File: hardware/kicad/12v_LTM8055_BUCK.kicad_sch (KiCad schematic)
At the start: 20 parts, among them U44 MCP4725A0T-E/CH, U47 LTM8055IY_PBF

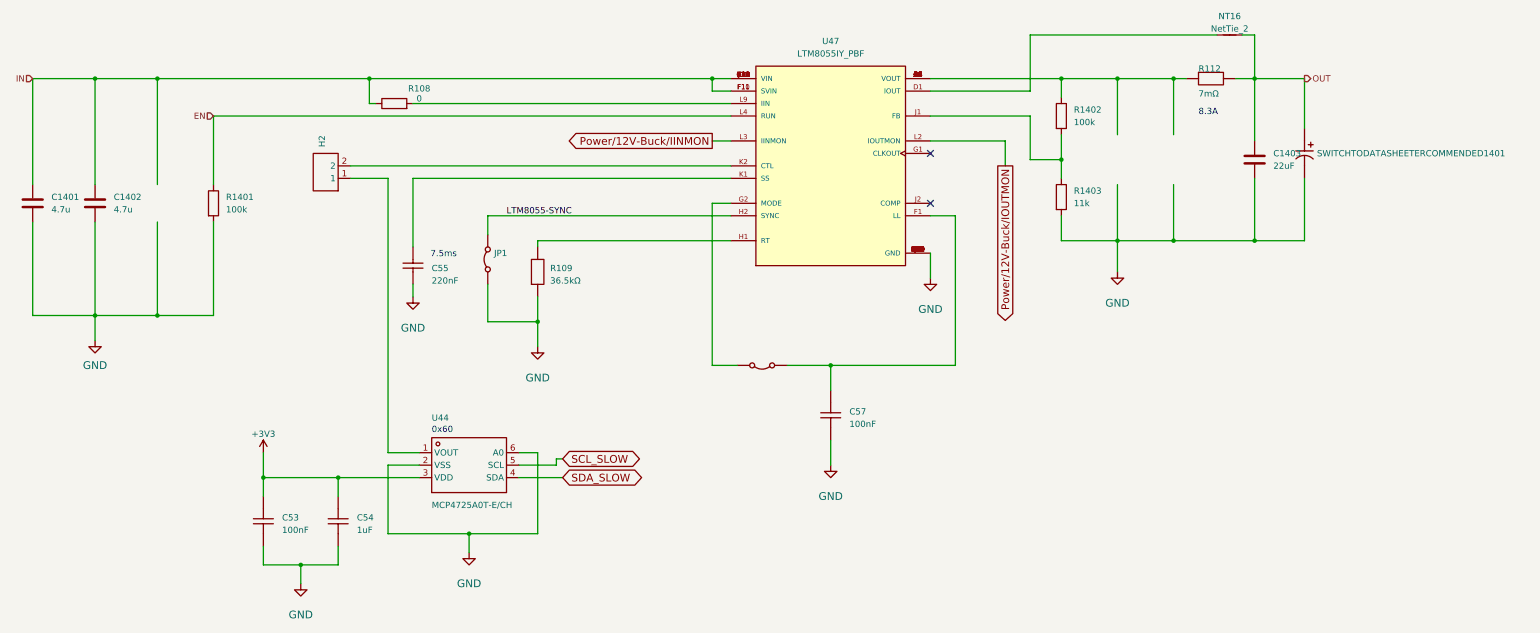
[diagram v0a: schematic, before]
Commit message: almost done 12v buck
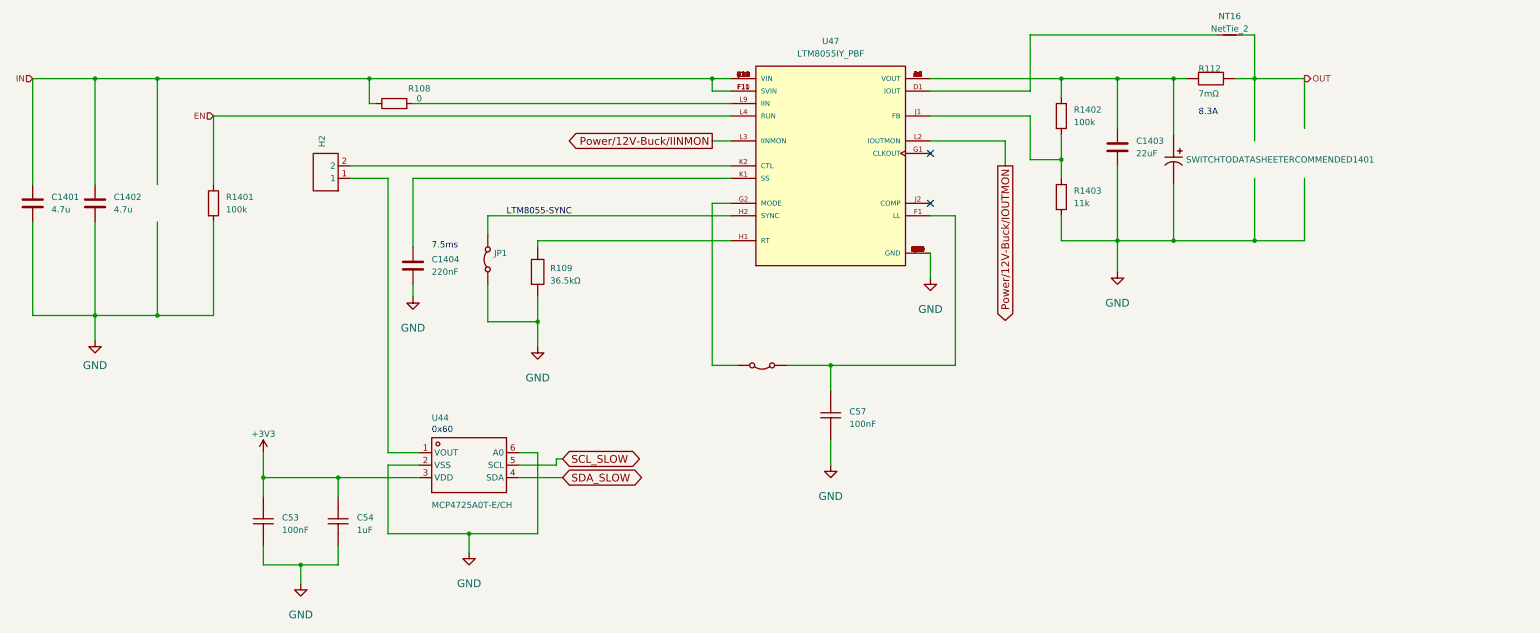
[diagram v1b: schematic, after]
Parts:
- removed C55: 220nF, 5v rail sm-easyedapro:C0603, symbol 5v rail sm-easyedapro:CL10B224KB8NNNC
- added C1404: 220nF, Capacitor_SMD:C_0402_1005Metric, symbol Device:C
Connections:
- net GND: now also C1404.2
- net OUT: no longer C1403.1, SWITCHTODATASHEETERCOMMENDED1401.1
- net at U47.K1 (SS): now also C1404.1
- net at R112.1, R1402.1, U47.A1 (VOUT)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: now also C1403.1, SWITCHTODATASHEETERCOMMENDED1401.1
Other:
- moved on the sheet: C1403, SWITCHTODATASHEETERCOMMENDED1401
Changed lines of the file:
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@@
 	(text "7.5ms"
 		(exclude_from_sim no)
-		(at 98.806 102.616 0)
+		(at 99.06 100.838 0)
 		(effects
 			(font
@@
 	(wire
 		(pts
-			(xy 238.76 87.63) (xy 238.76 99.06)
+			(xy 238.76 83.82) (xy 238.76 99.06)
 		)
 		(stroke
@@
 	(wire
 		(pts
-			(xy 238.76 66.04) (xy 238.76 77.47)
+			(xy 238.76 66.04) (xy 238.76 76.2)
 		)
 		(stroke
@@
 	)
 	(symbol
-		(lib_id "5v rail sm-easyedapro:CL10B224KB8NNNC")
-		(at 95.25 104.14 90)
-		(unit 1)
-		(exclude_from_sim no)
-		(in_bom yes)
-		(on_board yes)
-		(dnp no)
-		(property "Reference" "C55"
-			(at 99.06 105.41 90)
-			(effects
-				(font
-					(size 1.27 1.27)
-				)
-				(justify right top)
-			)
-		)
-		(property "Value" "220nF"
-			(at 99.06 107.95 90)
-			(effects
-				(font
-					(size 1.27 1.27)
-				)
-				(justify right top)
-			)
-		)
-		(property "Footprint" "5v rail sm-easyedapro:C0603"
-			(at 95.25 104.14 0)
-			(effects
-				(font
-					(size 1.27 1.27)
-				)
-				(hide yes)
-			)
-		)
-		(property "Datasheet" "https://item.szlcsc.com/datasheet/CL10B224KB8NNNC/65773.html"
-			(at 95.25 104.14 0)
-			(effects
-				(font
-					(size 1.27 1.27)
-				)
-				(hide yes)
-			)
-		)
-		(property "Description" "Capacitance:220nF Tolerance:±10% Tolerance:±10% Voltage Rating:50V Temperature Coefficient:X7R"
-			(at 95.25 104.14 0)
-			(effects
-				(font
-					(size 1.27 1.27)
-				)
-				(hide yes)
-			)
-		)
-		(property "Manufacturer Part" "CL10B224KB8NNNC"
-			(at 95.25 104.14 0)
-			(effects
-				(font
-					(size 1.27 1.27)
-				)
-				(hide yes)
-			)
-		)
-		(property "Manufacturer" "SAMSUNG(三星)"
-			(at 95.25 104.14 0)
-			(effects
-				(font
-					(size 1.27 1.27)
-				)
-				(hide yes)
-			)
-		)
-		(property "Supplier Part" "C64705"
-			(at 95.25 104.14 0)
-			(effects
-				(font
-					(size 1.27 1.27)
-				)
-				(hide yes)
-			)
-		)
-		(property "Supplier" "LCSC"
-			(at 95.25 104.14 0)
-			(effects
-				(font
-					(size 1.27 1.27)
-				)
-				(hide yes)
-			)
-		)
-		(property "LCSC Part Name" "220nF ±10% 50V"
-			(at 95.25 104.14 0)
-			(effects
-				(font
-					(size 1.27 1.27)
-				)
-				(hide yes)
-			)
-		)
-		(pin "1"
-		)
-		(pin "2"
-		)
-		(instances
-			(project "svea_powerboard_rev3"
-				(path "/3f85abf4-0b95-4c4a-b7e9-06f59ca1ea3d/5c2e021f-c2d4-49e2-8c36-9a64f1f12001/535c4b9d-dd70-4891-8336-b5700298b4d1"
-					(reference "C55")
-					(unit 1)
-				)
-			)
-		)
-	)
-	(symbol
 		(lib_id "Device:NetTie_2")
 		(at 261.62 57.15 0)
@@
 	(symbol
 		(lib_id "5v rail sm-easyedapro:RVT1E680M0605")
-		(at 276.86 81.28 270)
+		(at 250.19 82.55 270)
 		(unit 1)
 		(exclude_from_sim no)
@@
 		(fields_autoplaced yes)
 		(property "Reference" "SWITCHTODATASHEETERCOMMENDED1401"
-			(at 279.4 81.2799 90)
+			(at 252.73 82.5499 90)
 			(effects
 				(font
@@
 		)
 		(property "Value" "68uF"
-			(at 276.86 81.28 0)
+			(at 250.19 82.55 0)
 			(effects
 				(font
@@
 		)
 		(property "Footprint" "5v rail sm-easyedapro:CAP-SMD_BD6.3-L6.6-W6.6-LS7.4-FD"
-			(at 276.86 81.28 0)
+			(at 250.19 82.55 0)
 			(effects
 				(font
@@
 		)
 		(property "Datasheet" ""
-			(at 276.86 81.28 0)
+			(at 250.19 82.55 0)
 			(effects
 				(font
@@
 		)
 		(property "Description" "Capacitance:68uF Tolerance:±20% Tolerance:±20% Voltage Rating:25V Ripple Current:55mA@120Hz Diameter:6.3mm Height - Seated (Max):5.4mm Lifetime:2000hrs@105°C Operating Temperature:-40°C~+105°C Operating Temperature:-40°C~+105°C"
-			(at 276.86 81.28 0)
+			(at 250.19 82.55 0)
 			(effects
 				(font
@@
 		)
 		(property "Manufacturer Part" "RVT1E680M0605"
-			(at 276.86 81.28 0)
+			(at 250.19 82.55 0)
 			(effects
 				(font
@@
 		)
 		(property "Manufacturer" "ROQANG(容强)"
-			(at 276.86 81.28 0)
+			(at 250.19 82.55 0)
 			(effects
 				(font
@@
 		)
 		(property "Supplier Part" "C7436903"
-			(at 276.86 81.28 0)
+			(at 250.19 82.55 0)
 			(effects
 				(font
@@
 		)
 		(property "Supplier" "LCSC"
-			(at 276.86 81.28 0)
+			(at 250.19 82.55 0)
 			(effects
 				(font
@@
 		)
 		(property "LCSC Part Name" "68uF ±20% 25V"
-			(at 276.86 81.28 0)
+			(at 250.19 82.55 0)
 			(effects
 				(font
@@
 		)
 		(instances
-			(project ""
+			(project "svea_powerboard_rev3"
 				(path "/3f85abf4-0b95-4c4a-b7e9-06f59ca1ea3d/5c2e021f-c2d4-49e2-8c36-9a64f1f12001/535c4b9d-dd70-4891-8336-b5700298b4d1"
 					(reference "SWITCHTODATASHEETERCOMMENDED1401")
@@
 	)
 	(symbol
+		(lib_id "Device:C")
+		(at 95.25 104.14 0)
+		(unit 1)
+		(exclude_from_sim no)
+		(in_bom yes)
+		(on_board yes)
+		(dnp no)
+		(fields_autoplaced yes)
+		(property "Reference" "C1404"
+			(at 99.06 102.8699 0)
+			(effects
+				(font
+					(size 1.27 1.27)
+				)
+				(justify left)
+			)
+		)
+		(property "Value" "220nF"
+			(at 99.06 105.4099 0)
+			(effects
+				(font
+					(size 1.27 1.27)
+				)
+				(justify left)
+			)
+		)
+		(property "Footprint" "Capacitor_SMD:C_0402_1005Metric"
+			(at 96.2152 107.95 0)
+			(effects
+				(font
+					(size 1.27 1.27)
+				)
+				(hide yes)
+			)
+		)
+		(property "Datasheet" "~"
+			(at 95.25 104.14 0)
+			(effects
+				(font
+					(size 1.27 1.27)
+				)
+				(hide yes)
+			)
+		)
+		(property "Description" "Unpolarized capacitor"
+			(at 95.25 104.14 0)
+			(effects
+				(font
+					(size 1.27 1.27)
+				)
+				(hide yes)
+			)
+		)
+		(pin "1"
+		)
+		(pin "2"
+		)
+		(instances
+			(project ""
+				(path "/3f85abf4-0b95-4c4a-b7e9-06f59ca1ea3d/5c2e021f-c2d4-49e2-8c36-9a64f1f12001/535c4b9d-dd70-4891-8336-b5700298b4d1"
+					(reference "C1404")
+					(unit 1)
+				)
+			)
+		)
+	)
+	(symbol
 		(lib_id "power:GND")
 		(at 72.39 168.91 0)
@@
 	(symbol
 		(lib_id "Device:C")
-		(at 266.7 82.55 0)
+		(at 238.76 80.01 0)
 		(unit 1)
 		(exclude_from_sim no)
@@
 		(fields_autoplaced yes)
 		(property "Reference" "C1403"
-			(at 270.51 81.2799 0)
+			(at 242.57 78.7399 0)
 			(effects
 				(font
@@
 		)
 		(property "Value" "22uF"
-			(at 270.51 83.8199 0)
+			(at 242.57 81.2799 0)
 			(effects
 				(font
@@
 		)
 		(property "Footprint" "Capacitor_SMD:C_0805_2012Metric"
-			(at 267.6652 86.36 0)
+			(at 239.7252 83.82 0)
 			(effects
 				(font
@@
 		)
 		(property "Datasheet" "~"
-			(at 266.7 82.55 0)
+			(at 238.76 80.01 0)
 			(effects
 				(font
@@
 		)
 		(property "Description" "Unpolarized capacitor"
-			(at 266.7 82.55 0)
+			(at 238.76 80.01 0)
 			(effects
 				(font
@@
 		)
 		(instances
-			(project ""
+			(project "svea_powerboard_rev3"
 				(path "/3f85abf4-0b95-4c4a-b7e9-06f59ca1ea3d/5c2e021f-c2d4-49e2-8c36-9a64f1f12001/535c4b9d-dd70-4891-8336-b5700298b4d1"
 					(reference "C1403")
